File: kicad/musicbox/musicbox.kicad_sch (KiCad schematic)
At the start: 8 parts

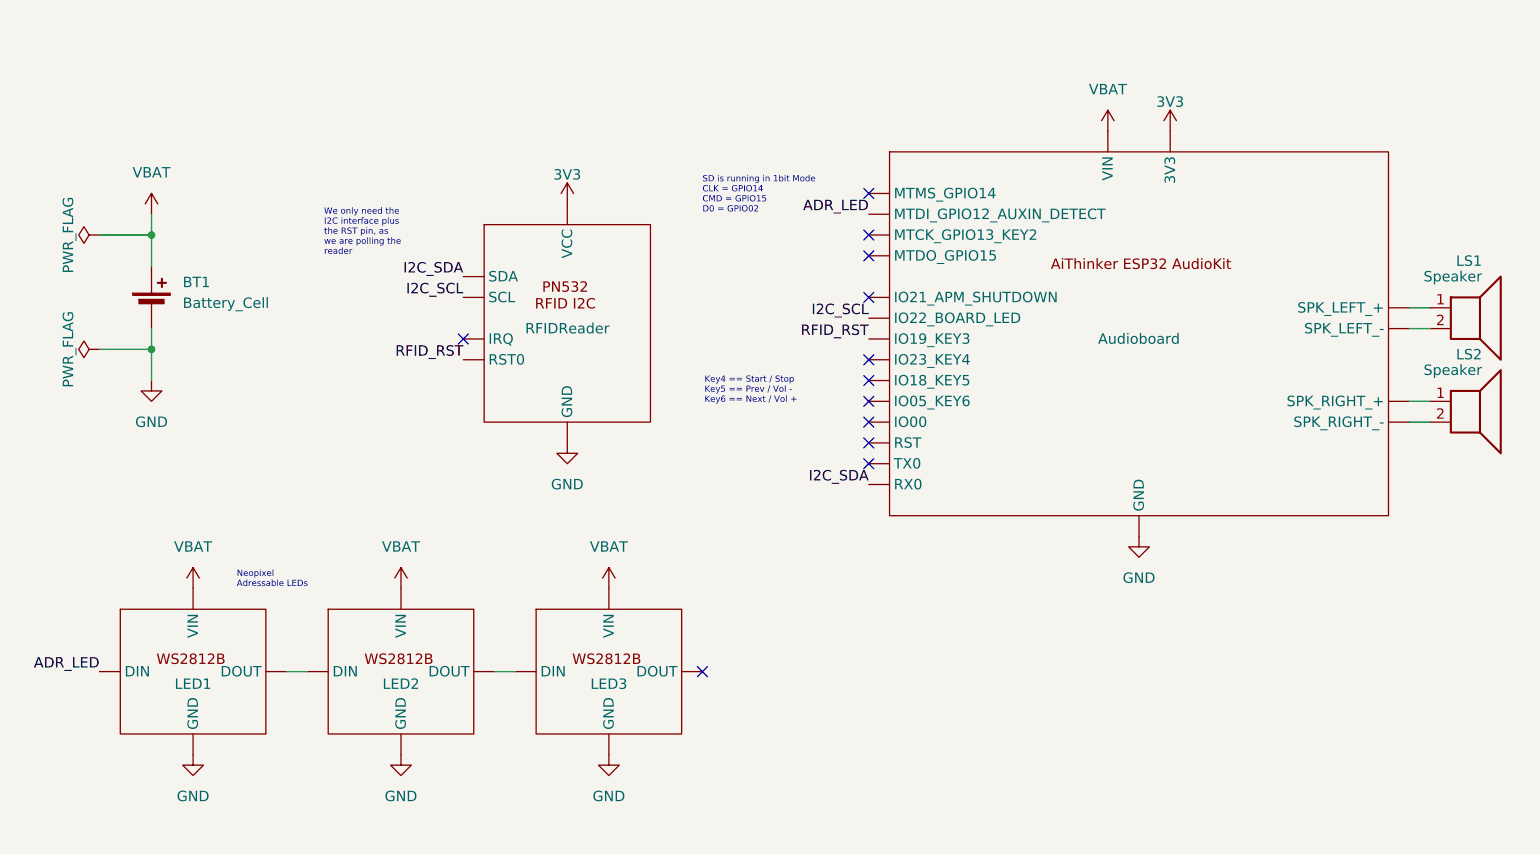
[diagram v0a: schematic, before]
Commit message: Updated the documentation
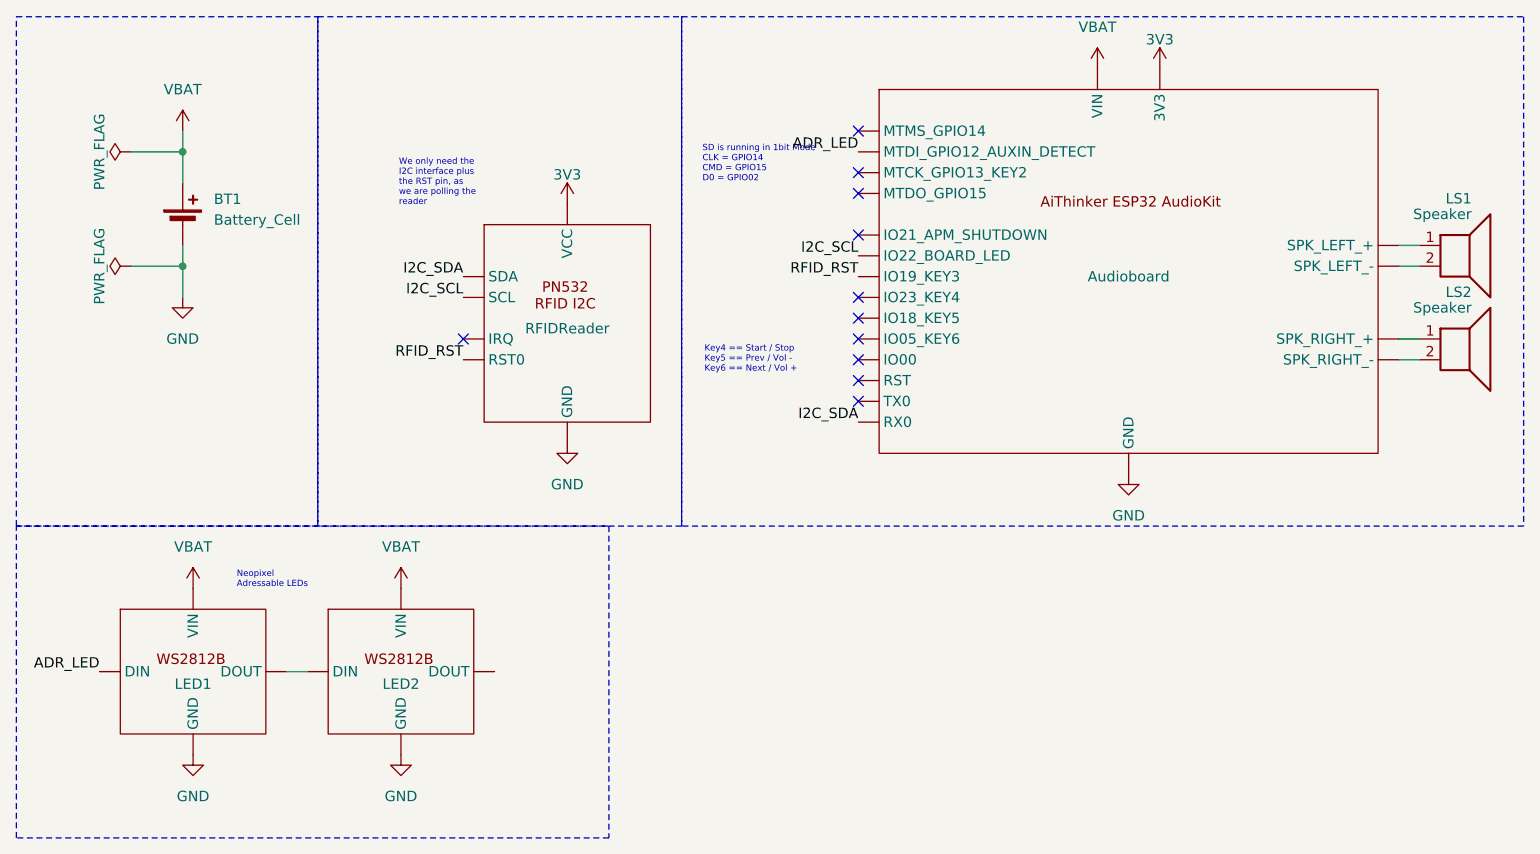
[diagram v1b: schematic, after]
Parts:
- removed LED3: ~, symbol custom_parts:WS2812B
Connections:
- new net: LED1. (VIN), LED2. (VIN)
- no-connect marks 12 -> 11
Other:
- moved on the sheet: Audioboard, BT1, LS1, LS2

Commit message: Working on newer prototype
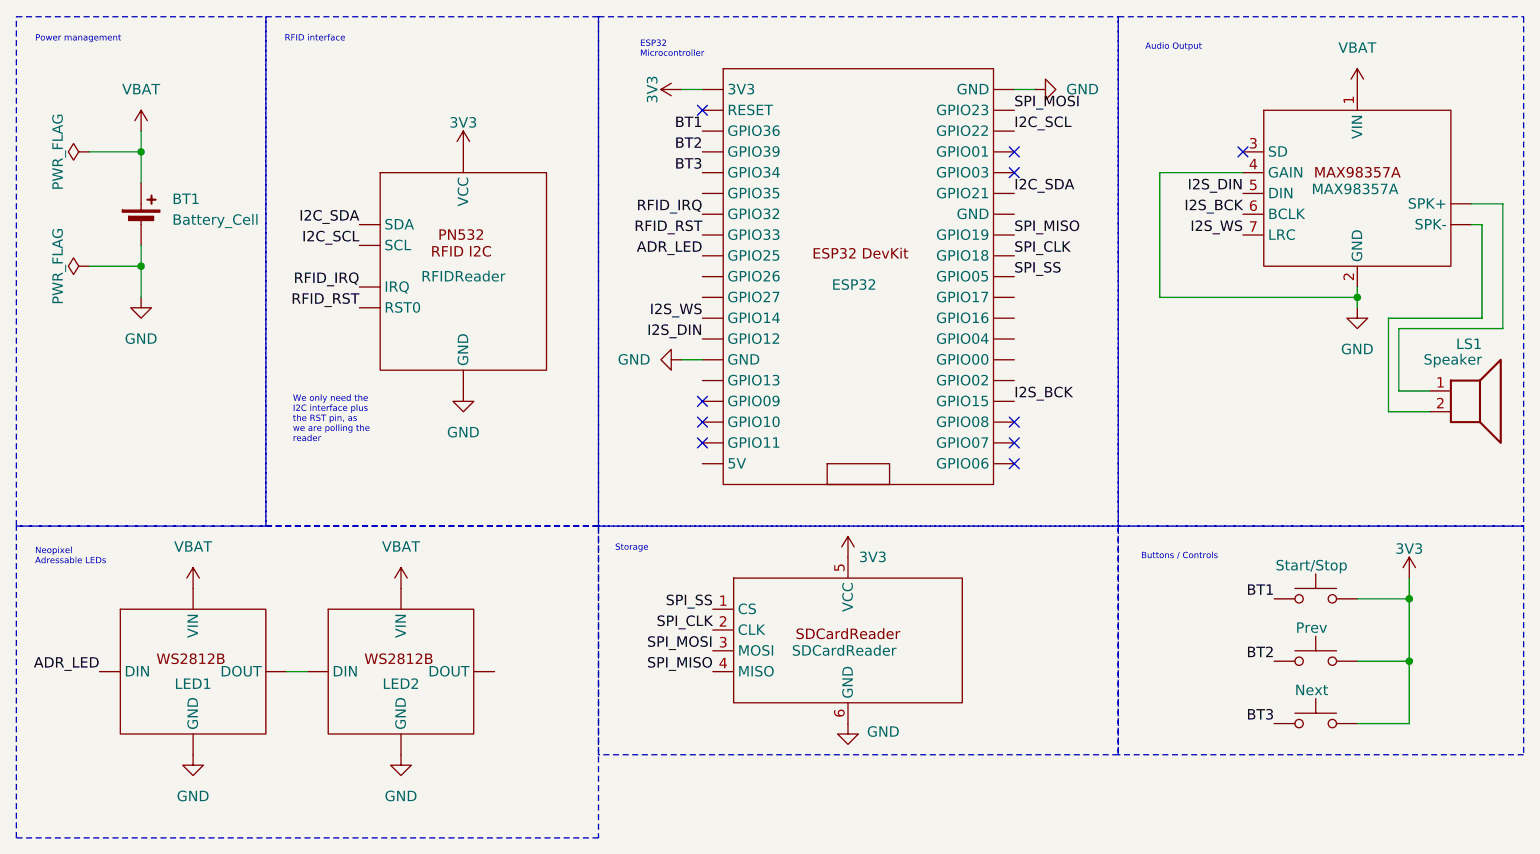
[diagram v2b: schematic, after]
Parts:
- removed Audioboard: ~, symbol custom_parts:AiThinker_ESP32_AudioKit
- removed LS2: Speaker, symbol Device:Speaker
- added ESP32: ~, symbol custom_parts:ESP32_DevKitC
- added MAX98357A: ~, symbol custom_parts:MAX98357A
- added Next, Prev, Start/Stop: Button, symbol Switch:SW_Push
- added SDCardReader: ~, symbol custom_parts:SDCardReader
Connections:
- net 3V3: now also ESP32. (GPIO06), Next.2, Prev.2, SDCardReader.5 (VCC), Start/Stop.2
- net ADR_LED: now also ESP32. (GPIO06)
- net GND: now also ESP32. (GPIO06), MAX98357A.2 (GND), MAX98357A.4 (GAIN), SDCardReader.6 (GND)
- net I2C_SCL: now also ESP32. (GPIO06)
- net I2C_SDA: now also ESP32. (GPIO06)
- net RFID_RST: now also ESP32. (GPIO06)
- net VBAT: now also MAX98357A.1 (VIN)
- net at LS1.1: now also MAX98357A. (SPK-)
- net at LS1.2: now also MAX98357A. (SPK-)
- new net: LED1. (DOUT), LED2. (DOUT)
- new net BT1: ESP32. (GPIO06), Start/Stop.1
- new net BT2: ESP32. (GPIO06), Prev.1
- new net BT3: ESP32. (GPIO06), Next.1
- new net I2S_BCK: ESP32. (GPIO06), MAX98357A.6 (BCLK)
- new net I2S_DIN: ESP32. (GPIO06), MAX98357A.5 (DIN)
- new net I2S_WS: ESP32. (GPIO06), MAX98357A.7 (LRC)
- new net RFID_IRQ: ESP32. (GPIO06), RFIDReader. (GND)
- new net SPI_CLK: ESP32. (GPIO06), SDCardReader.2 (CLK)
- new net SPI_MISO: ESP32. (GPIO06), SDCardReader.4 (MISO)
- new net SPI_MOSI: ESP32. (GPIO06), SDCardReader.3 (MOSI)
- new net SPI_SS: ESP32. (GPIO06), SDCardReader.1 (CS)
- no-connect marks 11 -> 10
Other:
- note added: "Audio Output"
- note added: "Buttons / Controls"
- note added: "ESP32 Microcontroller"
- note added: "Power management"
- note added: "RFID interface"
- note added: "Storage"
- note removed: "Key4 == Start / Stop Key5 == Prev / Vol - Key6 == Next / Vol +"
- note removed: "SD is running in 1bit Mode CLK = GPIO14 CMD = GPIO15 D0 = GPIO02"
- moved on the sheet: BT1, LS1, RFIDReader
